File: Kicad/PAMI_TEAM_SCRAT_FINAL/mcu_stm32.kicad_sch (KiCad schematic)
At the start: 13 parts, among them SW4 RESET, U1 STM32H573RITx, U2 STLINK-V3MODS

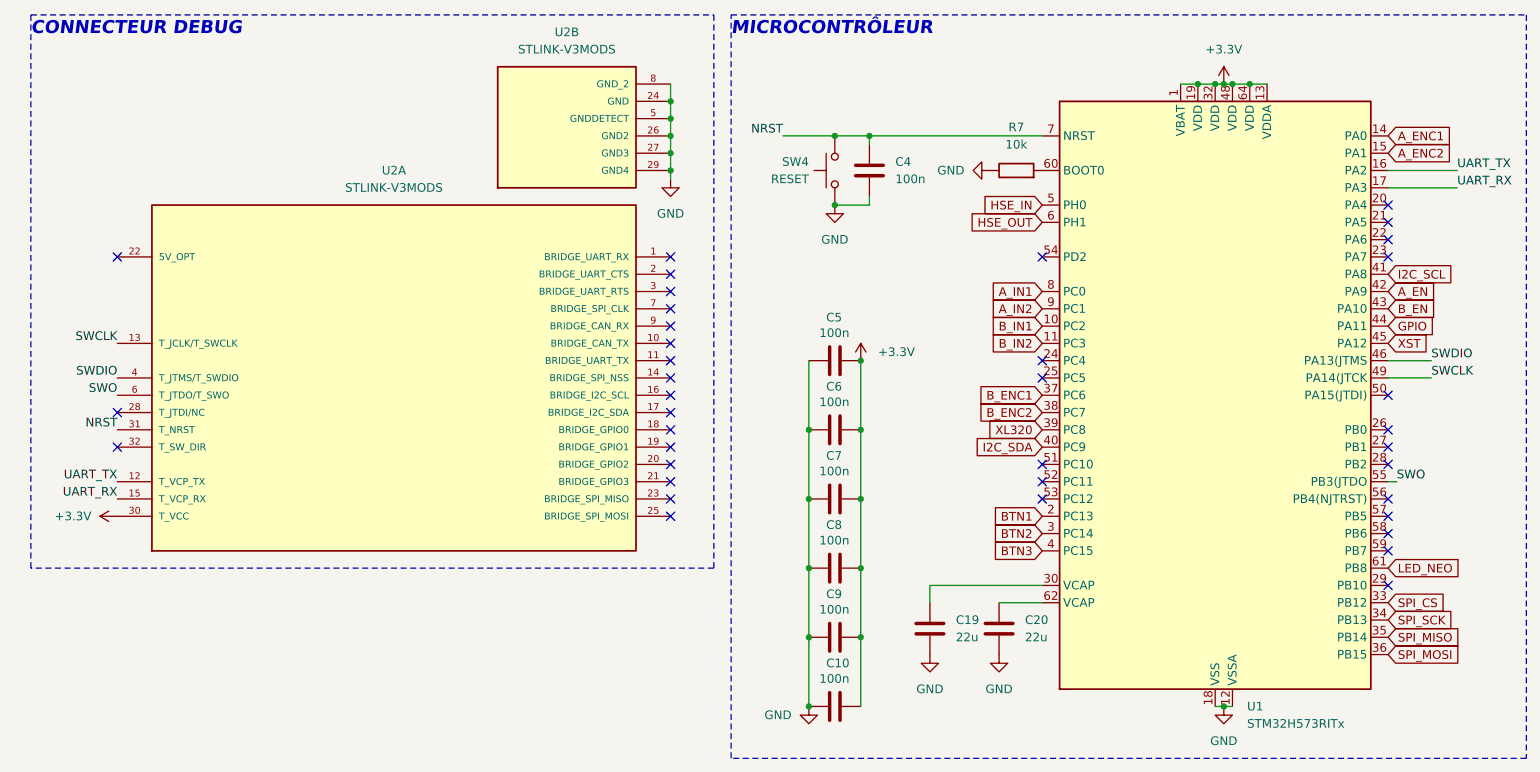
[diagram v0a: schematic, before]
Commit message: pcb termine
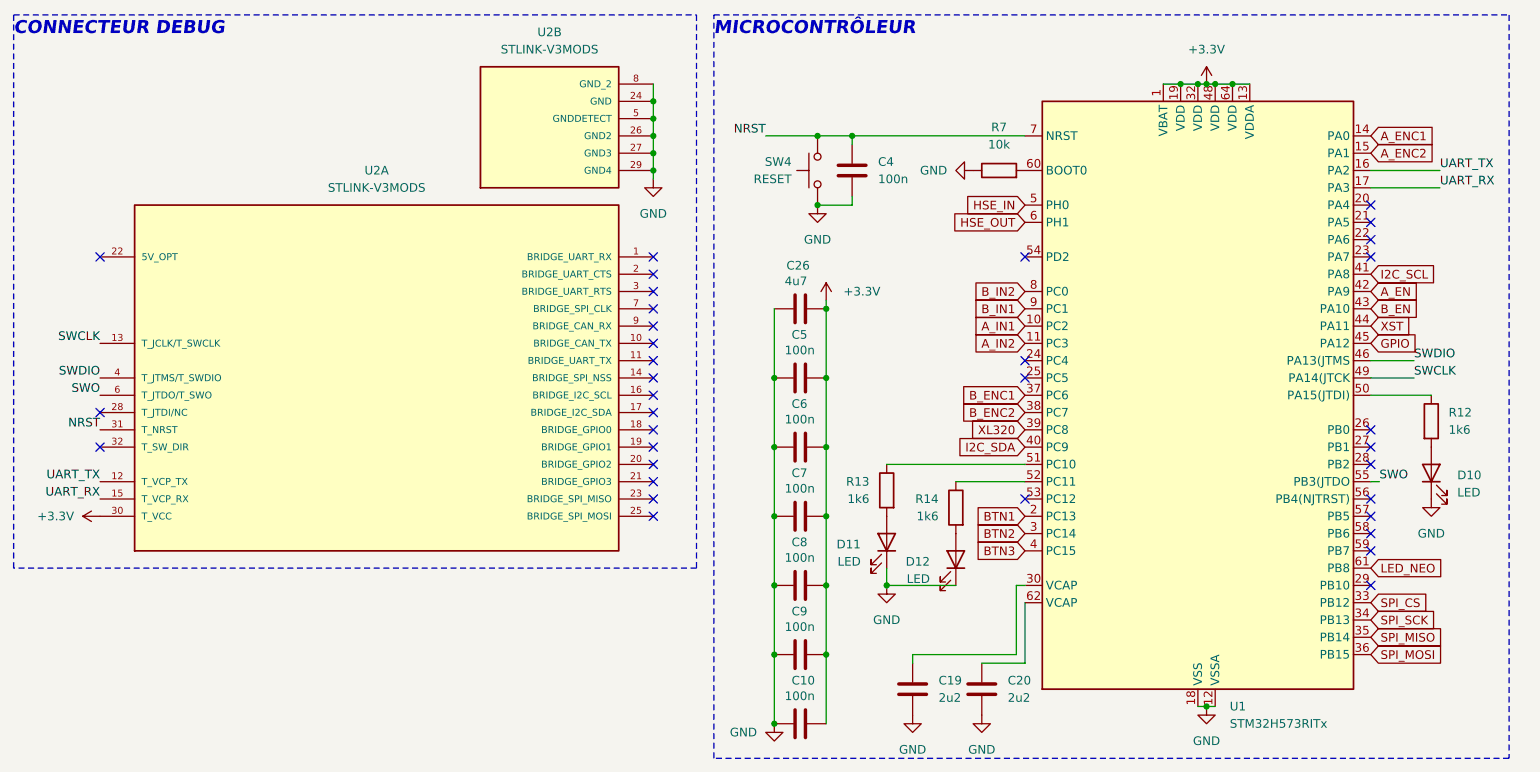
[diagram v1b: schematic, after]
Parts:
- added C26: 4u7, Capacitor_SMD:C_0402_1005Metric, symbol Device:C
- added D10, D11, D12: LED, LED_SMD:LED_0603_1608Metric, symbol Device:LED
- added R12, R13, R14: 1k6, Resistor_SMD:R_0603_1608Metric, symbol Device:R
- C10, C5, C6, C7, C8, C9: footprint Capacitor_SMD:C_0603_1608Metric -> Capacitor_SMD:C_0402_1005Metric
- C19, C20: value 22u -> 2u2; footprint Capacitor_SMD:C_0805_2012Metric -> Capacitor_SMD:C_0603_1608Metric
- SW4: footprint Button_Switch_SMD:Panasonic_EVQPUJ_EVQPUA -> Button_Switch_SMD:SW_SPST_PTS645Sx43SMTR92
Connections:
- net +3.3V: now also C26.2
- net A_IN1: now also U1.10 (PC2); no longer U1.8 (PC0)
- net A_IN2: now also U1.11 (PC3); no longer U1.9 (PC1)
- net B_IN1: now also U1.9 (PC1); no longer U1.10 (PC2)
- net B_IN2: now also U1.8 (PC0); no longer U1.11 (PC3)
- net GND: now also C26.1, D10.1 (K), D11.1 (K), D12.1 (K)
- net GPIO: now also U1.45 (PA12); no longer U1.44 (PA11)
- net XST: now also U1.44 (PA11); no longer U1.45 (PA12)
- net at U1.50 (PA15(JTDI)): now also R12.1
- net at U1.51 (PC10): now also R13.1
- net at U1.52 (PC11): now also R14.1
- new net: D11.2 (A), R13.2
- new net: D12.2 (A), R14.2
- new net: D10.2 (A), R12.2
- no-connect marks 38 -> 35
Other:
- moved on the sheet: C10, C19, C4, C5, C6, C7, C8, C9, R7, SW4, U1, U2A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
